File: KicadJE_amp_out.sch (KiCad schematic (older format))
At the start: 32 parts, among them J301 Tone/Noise, J302 RND, J303 TONE, J304 DRUM_OUT, J305 Tones, J306 Noise, U101 74HC04, U302 TL072

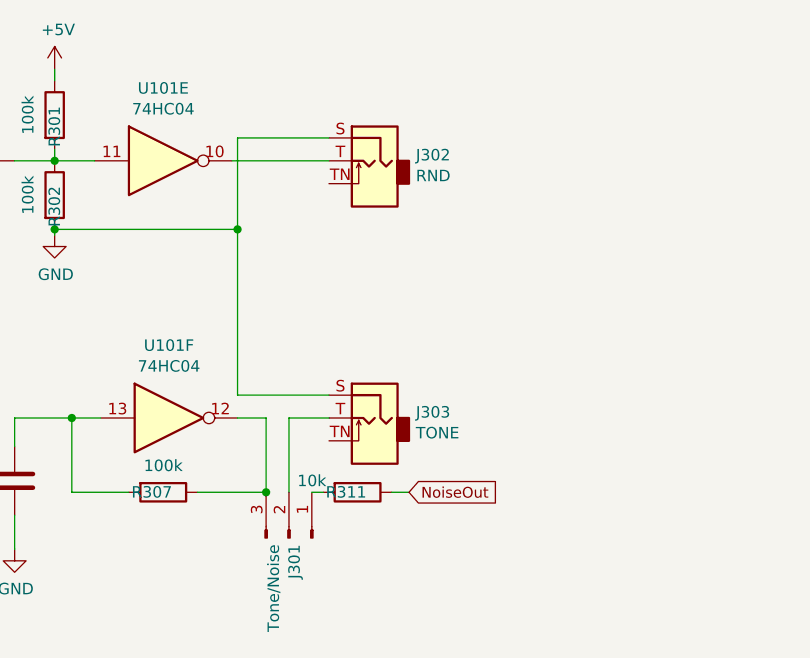
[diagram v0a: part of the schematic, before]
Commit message: AC coupled noise
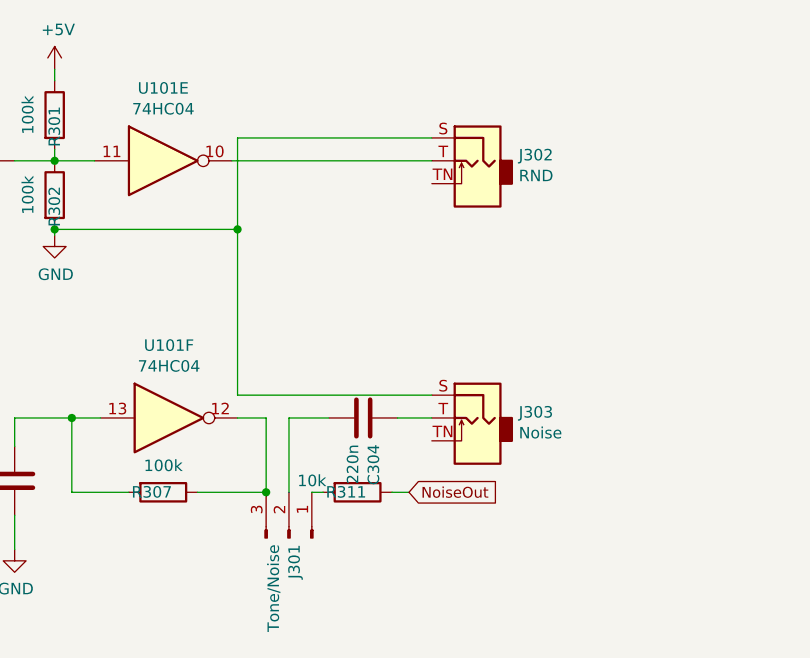
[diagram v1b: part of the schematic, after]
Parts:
- added C304: 220n, AJ:C_0805_AJ, symbol Device:C
- J303: value TONE -> Noise
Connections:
- net at J303.T: now also C304.1; no longer J301.2 (Pin_2)
- new net: C304.2, J301.2 (Pin_2)
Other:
- moved on the sheet: J302, J303
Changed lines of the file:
@@
 L Connector:AudioJack2_SwitchT J?
 U 1 1 61681759
-P 2800 1100
+P 3250 1100
 AR Path="/607E07E1/61681759" Ref="J?"  Part="1"
 AR Path="/61681759" Ref="J?"  Part="1"
 AR Path="/6165D4D0/61681759" Ref="J302"  Part="1"
-F 0 "J302" H 2620 1125 50  0000 R CNN
-F 1 "RND" H 2620 1034 50  0000 R CNN
-F 2 "Connector_Audio:Jack_3.5mm_QingPu_WQP-PJ398SM_Vertical_CircularHoles" H 2800 1100 50  0001 C CNN
-F 3 "~" H 2800 1100 50  0001 C CNN
-	1    2800 1100
+F 0 "J302" H 3070 1125 50  0000 R CNN
+F 1 "RND" H 3070 1034 50  0000 R CNN
+F 2 "Connector_Audio:Jack_3.5mm_QingPu_WQP-PJ398SM_Vertical_CircularHoles" H 3250 1100 50  0001 C CNN
+F 3 "~" H 3250 1100 50  0001 C CNN
+	1    3250 1100
 	-1   0    0    -1
 $EndComp
@@
 L Connector:AudioJack2_SwitchT J?
 U 1 1 61A8618F
-P 2800 2225
+P 3250 2225
 AR Path="/607E07E1/61A8618F" Ref="J?"  Part="1"
 AR Path="/61A8618F" Ref="J?"  Part="1"
 AR Path="/6165D4D0/61A8618F" Ref="J303"  Part="1"
-F 0 "J303" H 2620 2250 50  0000 R CNN
-F 1 "TONE" H 2620 2159 50  0000 R CNN
-F 2 "Connector_Audio:Jack_3.5mm_QingPu_WQP-PJ398SM_Vertical_CircularHoles" H 2800 2225 50  0001 C CNN
-F 3 "~" H 2800 2225 50  0001 C CNN
-	1    2800 2225
+F 0 "J303" H 3070 2250 50  0000 R CNN
+F 1 "Noise" H 3070 2159 50  0000 R CNN
+F 2 "Connector_Audio:Jack_3.5mm_QingPu_WQP-PJ398SM_Vertical_CircularHoles" H 3250 2225 50  0001 C CNN
+F 3 "~" H 3250 2225 50  0001 C CNN
+	1    3250 2225
 	-1   0    0    -1
 $EndComp
-Wire Wire Line
-	2200 1000 2600 1000
-Wire Wire Line
-	2175 1100 2600 1100
-Wire Wire Line
-	2600 2125 2200 2125
 Wire Wire Line
 	2200 2125 2200 1400
@@
 	4325 4200 5000 4200
 Connection ~ 4325 4200
+$Comp
+L Device:C C?
+U 1 1 6089BC96
+P 2750 2225
+AR Path="/6089BC96" Ref="C?"  Part="1"
+AR Path="/6165D4D0/6089BC96" Ref="C304"  Part="1"
+F 0 "C304" H 2865 2271 50  0000 L CNN
+F 1 "220n" H 2865 2180 50  0000 L CNN
+F 2 "AJ:C_0805_AJ" H 2788 2075 50  0001 C CNN
+F 3 "~" H 2750 2225 50  0001 C CNN
+	1    2750 2225
+	0    1    1    0
+$EndComp
+Wire Wire Line
+	2900 2225 3050 2225
+Wire Wire Line
+	2200 2125 3050 2125
+Wire Wire Line
+	2175 1100 3050 1100
+Wire Wire Line
+	2200 1000 3050 1000
 $EndSCHEMATC
